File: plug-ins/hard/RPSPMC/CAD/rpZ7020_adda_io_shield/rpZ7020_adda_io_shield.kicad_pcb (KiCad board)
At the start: 4 copper layers, 61.3 x 89.9 mm, 24 parts, among them J1 Samtec_ASP-134486-01, J2-FMC-RP1 Conn_02x20, J3-FMC-POWER1 Conn_02x06_Odd_Even, J4-FMC-AUX1 Conn_02x06_Odd_Even

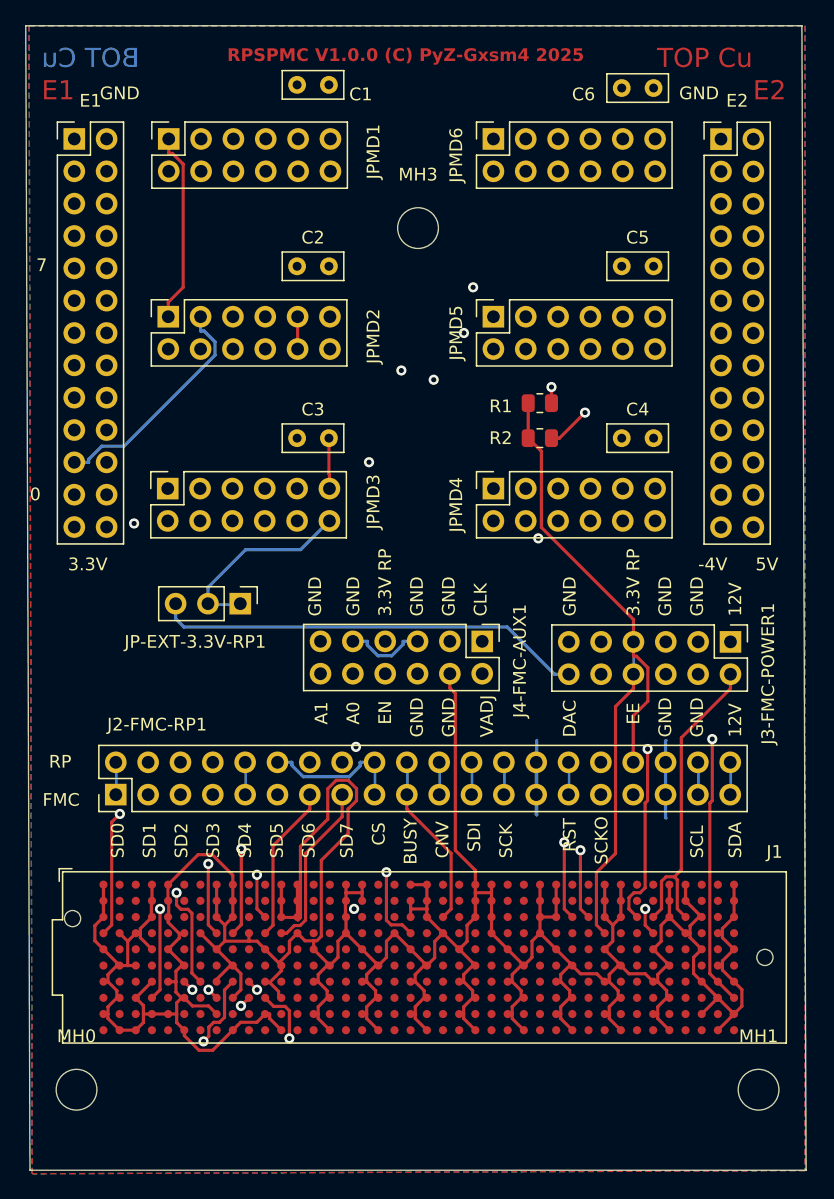
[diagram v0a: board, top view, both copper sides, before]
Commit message: fine tune brd
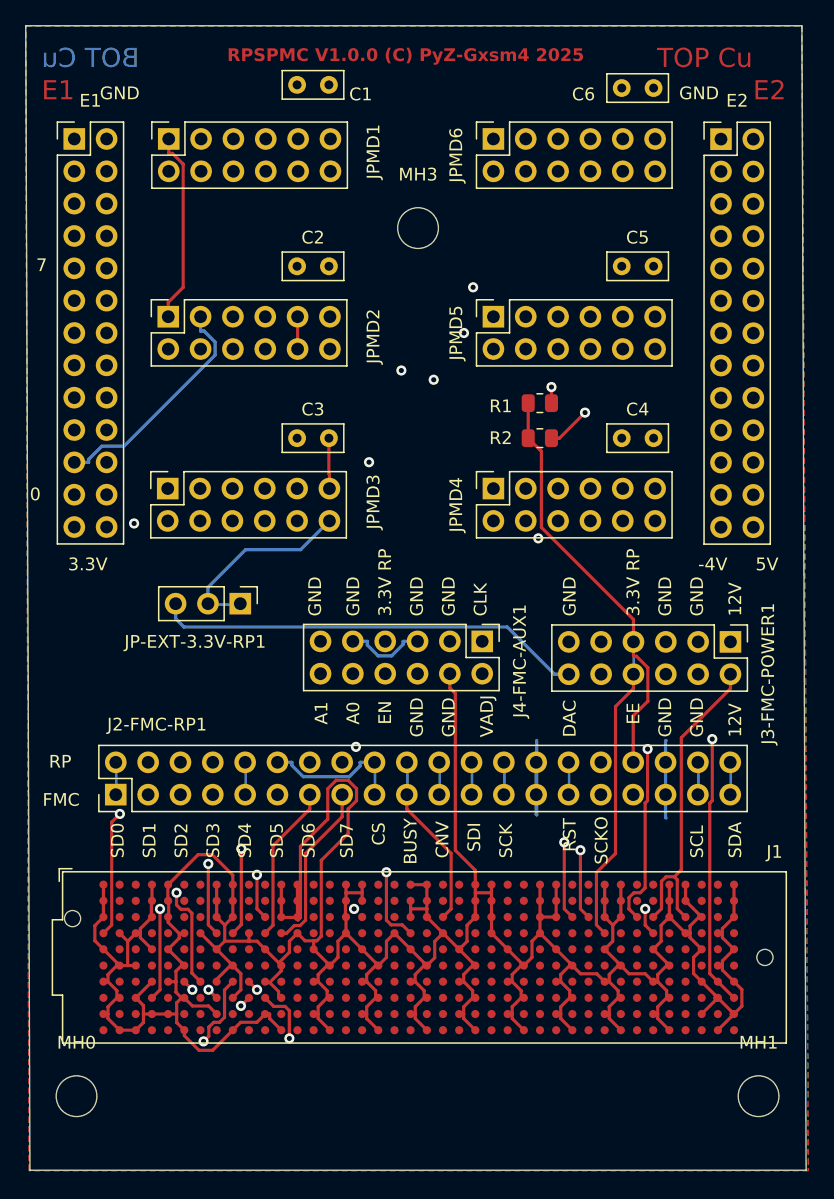
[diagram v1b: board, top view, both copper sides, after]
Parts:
- moved MH0 0.51 mm to (122.1, 159.0)
- moved MH1 0.51 mm to (175.7, 159.0)
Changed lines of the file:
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@@
 	(footprint "MountingHole:MountingHole_3.2mm_M3"
 		(layer "F.Cu")
-		(at 175.6614 158.511)
+		(at 175.6614 159.019)
 		(descr "Mounting Hole 3.2mm, no annular, M3")
 		(tags "mounting hole 3.2mm no annular m3")
@@
 	(footprint "MountingHole:MountingHole_3.2mm_M3"
 		(layer "F.Cu")
-		(at 122.0928 158.511)
+		(at 122.0928 159.019)
 		(descr "Mounting Hole 3.2mm, no annular, M3")
 		(tags "mounting hole 3.2mm no annular m3")
@@
 		(polygon
 			(pts
-				(xy 118.359 74.945) (xy 179.319 74.945) (xy 179.319 164.861) (xy 118.613 165.115)
+				(xy 118.105 74.945) (xy 179.065 74.945) (xy 179.573 164.861) (xy 118.359 164.861)
 			)
 		)
